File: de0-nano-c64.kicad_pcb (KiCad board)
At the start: 2 copper layers, 71.6 x 84 mm, 52 parts, among them J1 GPIO_0, J10 SD_Card, J2 PS2_0, J3 PS2_1, J4 AUDIO_L, J5 GPIO_1, J6 VGA_OUT, J7 AUDIO_R, J8 JOYSTICK_1, J9 JOYSTICK_2

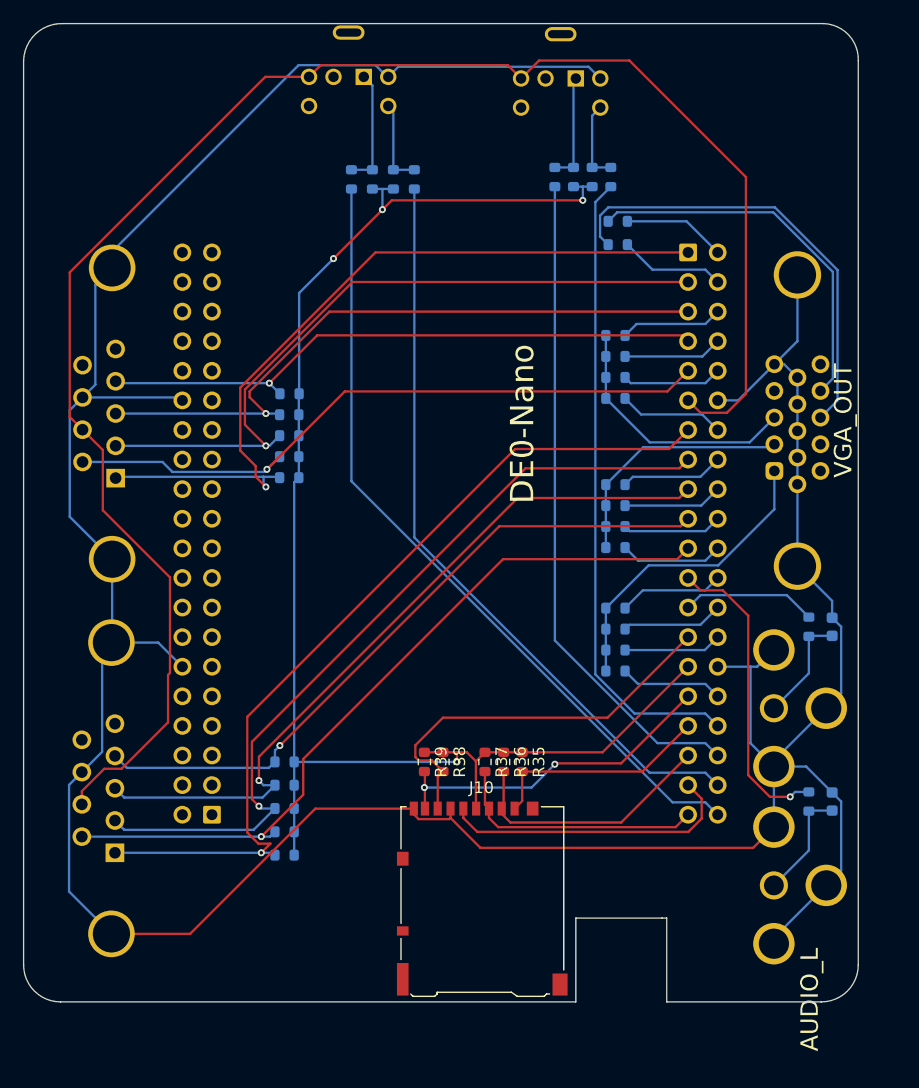
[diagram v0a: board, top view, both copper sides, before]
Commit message: .
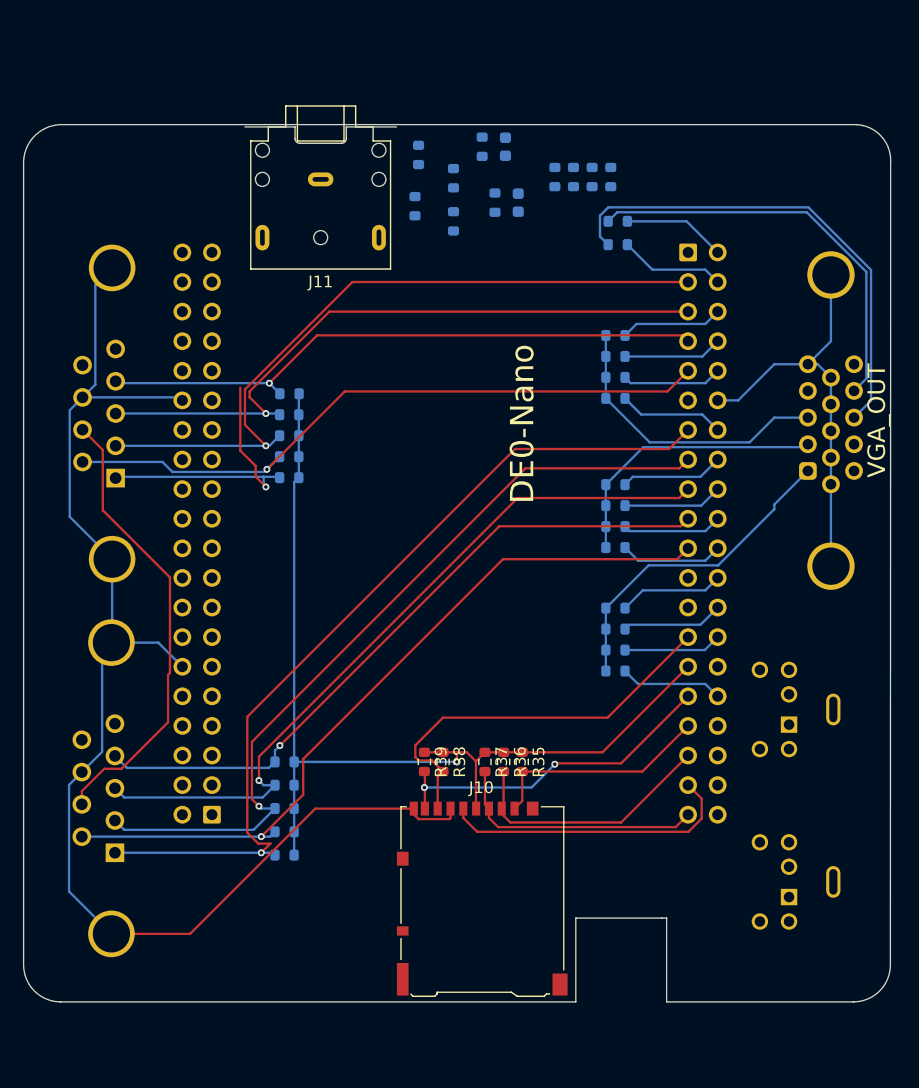
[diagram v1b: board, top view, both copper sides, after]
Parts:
- removed J4: AUDIO_L, 000_LOCAL:RCA
- removed J7: AUDIO_R, 000_LOCAL:RCA
- added J11: AudioJack3, Connector_Audio:Jack_3.5mm_CUI_SJ1-3523N_Horizontal, F.Cu at (132.1, 70.6)
- moved J3 76.4 mm to (176.1, 130.9), turned to -90 degrees
- moved J2 71.5 mm to (176.1, 116.1), turned to -90 degrees
- moved C1 58.0 mm to (149.1, 72.6)
- moved R22 58.0 mm to (147.1, 72.6)
- moved C2 49.8 mm to (148.0, 67.8)
- moved R23 49.8 mm to (146.0, 67.8)
- moved R16 5.92 mm to (140.2, 72.9)
- moved R15 5.16 mm to (143.5, 70.5)
- moved R17 4.92 mm to (143.5, 74.2)
- moved R14 4.48 mm to (140.5, 68.5)
- moved J6 2.88 mm to (175.9, 91.3)
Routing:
- net GND: track 290.6 -> 150.1 mm
- net +5V: track 148.6 -> 39.3 mm
- net /PS2_0_DAT: track 68.4 -> 0.00 mm
- net /PS2_0_CLK: track 64.8 -> 0.00 mm
- net /PS2_1_DAT: track 57.0 -> 0.00 mm
- net /PS2_1_CLK: track 54.7 -> 0.00 mm
- net /J1_UP: track 67.8 -> 24.5 mm
- net +3V3: track 127.6 -> 85.0 mm, vias 4 -> 1
- net /PWM_L: track 26.3 -> 0.00 mm, vias 1 -> 0
- net /PWM_R: track 11.6 -> 0.00 mm
- net Net-(J2-Pad1): track 10.1 -> 0.00 mm
- net Net-(C1-Pad1): track 9.64 -> 0.07 mm
- net Net-(C2-Pad1): track 9.43 -> 0.07 mm
- net Net-(J3-Pad1): track 9.60 -> 0.28 mm
- net Net-(J2-Pad5): track 7.46 -> 0.00 mm
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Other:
- board size 71.6 x 84 mm -> 74.4 x 75.3 mm
